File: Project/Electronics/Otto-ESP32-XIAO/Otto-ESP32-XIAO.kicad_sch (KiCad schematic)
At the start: 29 parts, among them J1 Conn_01x03, J10 Conn_01x02, J11 Conn_01x04, J12 OLED 0,91" - I2C (SKU21796), J13 MPU6050, J2 Conn_01x03, J3 Conn_01x03, J4 Conn_01x03, J5 Conn_01x03, J6 Conn_01x03, J7 Conn_01x04, J8 PCA9685, J9 Conn_01x04, SW1 SW_SPDT, U1 MOUDLE-SEEEDUINO-XIAO-ESP32C3, U2 R-78E5.0-1.0, U3 TMC2208_SILENTSTEPSTICK, U4 TMC2208_SILENTSTEPSTICK

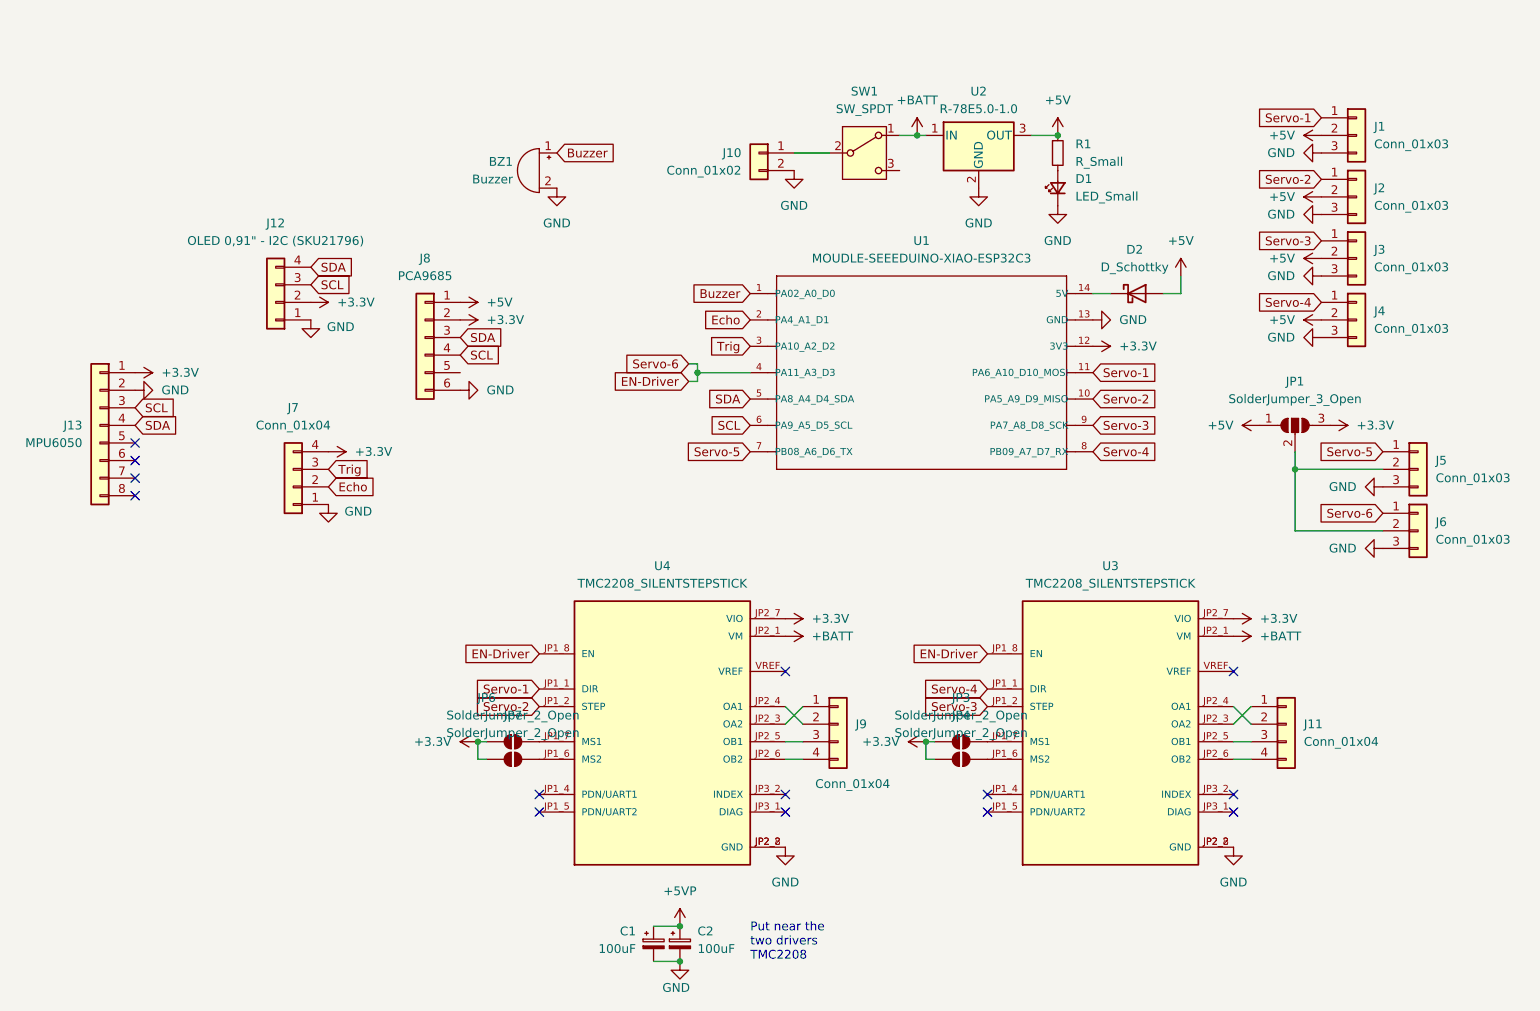
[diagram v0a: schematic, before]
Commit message: routing and documentation
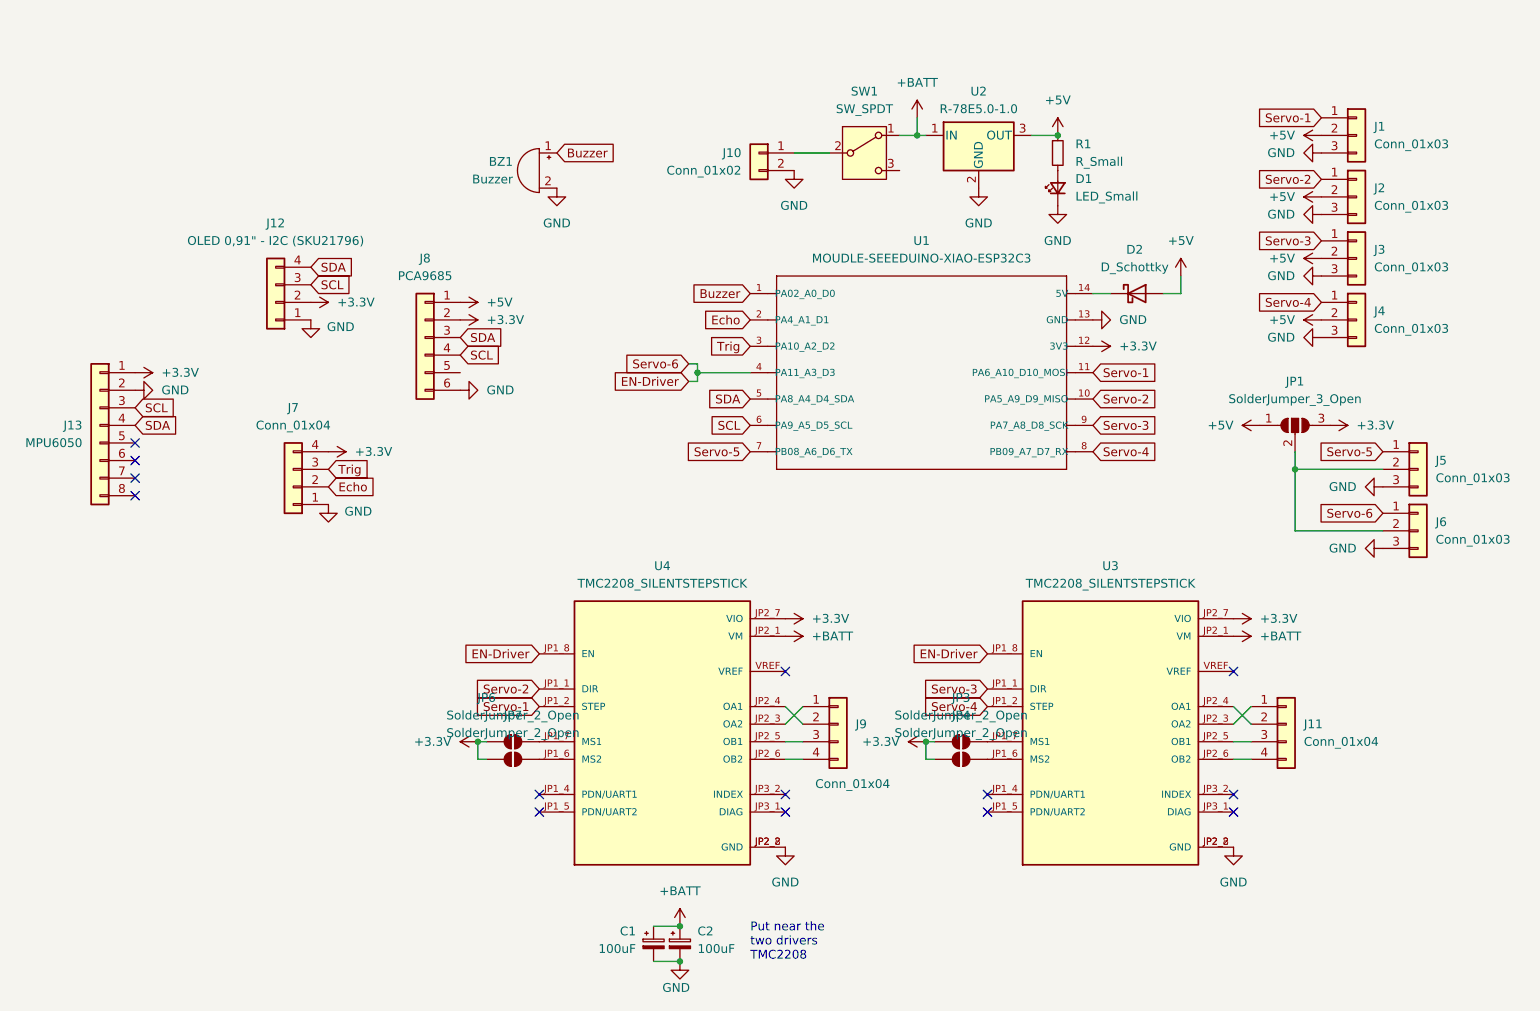
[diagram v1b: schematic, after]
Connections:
- net +5VP is gone; now on net +BATT: C1.1, C2.1
- net Servo-1: now also U4.JP1_2 (STEP); no longer U4.JP1_1 (DIR)
- net Servo-2: now also U4.JP1_1 (DIR); no longer U4.JP1_2 (STEP)
- net Servo-3: now also U3.JP1_1 (DIR); no longer U3.JP1_2 (STEP)
- net Servo-4: now also U3.JP1_2 (STEP); no longer U3.JP1_1 (DIR)
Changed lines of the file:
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@@
 	)
 	(junction
-		(at 111.76 168.91)
+		(at 114.3 88.9)
 		(diameter 0)
 		(color 0 0 0 0)
 	)
 	(junction
-		(at 114.3 88.9)
+		(at 200.66 102.87)
 		(diameter 0)
 		(color 0 0 0 0)
 	)
 	(junction
-		(at 200.66 102.87)
+		(at 146.05 54.61)
 		(diameter 0)
 		(color 0 0 0 0)
 	)
 	(junction
-		(at 146.05 54.61)
+		(at 111.76 168.91)
 		(diameter 0)
 		(color 0 0 0 0)
@@
 	(wire
 		(pts
-			(xy 146.05 54.61) (xy 147.32 54.61)
-		)
-		(stroke
-			(width 0)
-			(type default)
-		)
-	)
-	(wire
-		(pts
 			(xy 129.54 144.78) (xy 127 144.78)
 		)
@@
 	(wire
 		(pts
+			(xy 146.05 54.61) (xy 147.32 54.61)
+		)
+		(stroke
+			(width 0)
+			(type default)
+		)
+	)
+	(wire
+		(pts
 			(xy 147.32 142.24) (xy 147.32 144.78)
 		)
@@
 	(wire
 		(pts
+			(xy 143.51 54.61) (xy 146.05 54.61)
+		)
+		(stroke
+			(width 0)
+			(type default)
+		)
+	)
+	(wire
+		(pts
 			(xy 181.61 77.47) (xy 184.15 77.47)
 		)
@@
 	(wire
 		(pts
-			(xy 143.51 54.61) (xy 146.05 54.61)
+			(xy 107.95 168.91) (xy 111.76 168.91)
 		)
 		(stroke
@@
 	(wire
 		(pts
-			(xy 107.95 168.91) (xy 111.76 168.91)
+			(xy 191.77 139.7) (xy 194.31 137.16)
 		)
 		(stroke
@@
 	(wire
 		(pts
-			(xy 191.77 139.7) (xy 194.31 137.16)
+			(xy 114.3 88.9) (xy 114.3 90.17)
 		)
 		(stroke
@@
 	(wire
 		(pts
-			(xy 114.3 88.9) (xy 114.3 90.17)
+			(xy 200.66 111.76) (xy 200.66 102.87)
 		)
 		(stroke
@@
 	(wire
 		(pts
-			(xy 200.66 111.76) (xy 200.66 102.87)
+			(xy 82.55 144.78) (xy 83.82 144.78)
 		)
 		(stroke
@@
 	(wire
 		(pts
-			(xy 82.55 144.78) (xy 83.82 144.78)
+			(xy 191.77 137.16) (xy 194.31 139.7)
 		)
 		(stroke
@@
 	(wire
 		(pts
-			(xy 191.77 137.16) (xy 194.31 139.7)
+			(xy 146.05 52.07) (xy 146.05 54.61)
 		)
 		(stroke
@@
 		)
 	)
-	(global_label "Servo-4"
+	(global_label "Servo-3"
 		(shape input)
 		(at 156.21 134.62 180)
@@
 		)
 	)
-	(global_label "Servo-1"
+	(global_label "Servo-2"
 		(shape input)
 		(at 91.44 134.62 180)
@@
 		)
 	)
-	(global_label "Servo-2"
+	(global_label "Servo-1"
 		(shape input)
 		(at 91.44 137.16 180)
@@
 		)
 	)
-	(global_label "Servo-3"
+	(global_label "Servo-4"
 		(shape input)
 		(at 156.21 137.16 180)
@@
 	(symbol
 		(lib_id "power:+BATT")
-		(at 146.05 54.61 0)
+		(at 146.05 52.07 0)
 		(unit 1)
 		(exclude_from_sim no)
@@
 		(fields_autoplaced yes)
 		(property "Reference" "#PWR02"
-			(at 146.05 58.42 0)
+			(at 146.05 55.88 0)
 			(effects
 				(font
@@
 		)
 		(property "Value" "+BATT"
-			(at 146.05 49.53 0)
+			(at 146.05 46.99 0)
 			(effects
 				(font
@@
 		)
 		(property "Footprint" ""
-			(at 146.05 54.61 0)
+			(at 146.05 52.07 0)
 			(effects
 				(font
@@
 		)
 		(property "Datasheet" ""
-			(at 146.05 54.61 0)
+			(at 146.05 52.07 0)
 			(effects
 				(font
@@
 		)
 		(property "Description" "Power symbol creates a global label with name \"+BATT\""
-			(at 146.05 54.61 0)
+			(at 146.05 52.07 0)
 			(effects
 				(font
@@
 	)
 	(symbol
-		(lib_id "power:+5VP")
-		(at 111.76 168.91 0)
-		(unit 1)
-		(exclude_from_sim no)
-		(in_bom yes)
-		(on_board yes)
-		(dnp no)
-		(fields_autoplaced yes)
-		(property "Reference" "#PWR035"
-			(at 111.76 172.72 0)
-			(effects
-				(font
-					(size 1.27 1.27)
-				)
-				(hide yes)
-			)
-		)
-		(property "Value" "+5VP"
-			(at 111.76 163.83 0)
-			(effects
-				(font
-					(size 1.27 1.27)
-				)
-			)
-		)
-		(property "Footprint" ""
-			(at 111.76 168.91 0)
-			(effects
-				(font
-					(size 1.27 1.27)
-				)
-				(hide yes)
-			)
-		)
-		(property "Datasheet" ""
-			(at 111.76 168.91 0)
-			(effects
-				(font
-					(size 1.27 1.27)
-				)
-				(hide yes)
-			)
-		)
-		(property "Description" ""
-			(at 111.76 168.91 0)
-			(effects
-				(font
-					(size 1.27 1.27)
-				)
-				(hide yes)
-			)
-		)
-		(pin "1"
-		)
-		(instances
-			(project "Otto-ESP32-XIAO"
-				(path "/d2682c99-4285-4c0b-9e61-08b763b3ce0d"
-					(reference "#PWR035")
-					(unit 1)
-				)
-			)
-		)
-	)
-	(symbol
 		(lib_id "Connector_Generic:Conn_01x03")
 		(at 209.55 54.61 0)
@@
 					(unit 1)
 				)
+			)
+		)
+	)
+	(symbol
+		(lib_id "power:+BATT")
+		(at 111.76 168.91 0)
+		(unit 1)
+		(exclude_from_sim no)
+		(in_bom yes)
+		(on_board yes)
+		(dnp no)
+		(fields_autoplaced yes)
+		(property "Reference" "#PWR041"
+			(at 111.76 172.72 0)
+			(effects
+				(font
+					(size 1.27 1.27)
+				)
+				(hide yes)
+			)
+		)
+		(property "Value" "+BATT"
+			(at 111.76 163.83 0)
+			(effects
+				(font
+					(size 1.27 1.27)
+				)
+			)
+		)
+		(property "Footprint" ""
+			(at 111.76 168.91 0)
+			(effects
+				(font
+					(size 1.27 1.27)
+				)
+				(hide yes)
+			)
+		)
+		(property "Datasheet" ""
+			(at 111.76 168.91 0)
+			(effects
+				(font
+					(size 1.27 1.27)
+				)
+				(hide yes)
+			)
+		)
+		(property "Description" "Power symbol creates a global label with name \"+BATT\""
+			(at 111.76 168.91 0)
+			(effects
+				(font
+					(size 1.27 1.27)
+				)
+				(hide yes)
+			)
+		)
+		(pin "1"
+		)
+		(instances
+			(project "Otto-ESP32-XIAO"
+				(path "/d2682c99-4285-4c0b-9e61-08b763b3ce0d"
+					(reference "#PWR041")
+					(unit 1)
+				)

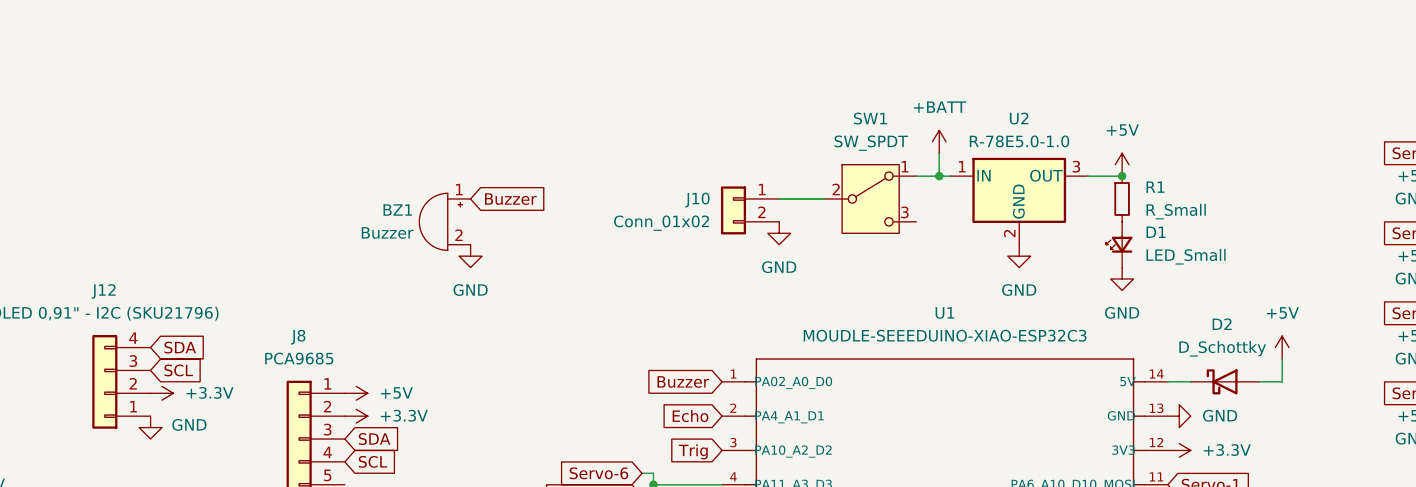
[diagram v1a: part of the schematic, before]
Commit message: New PCB lite version
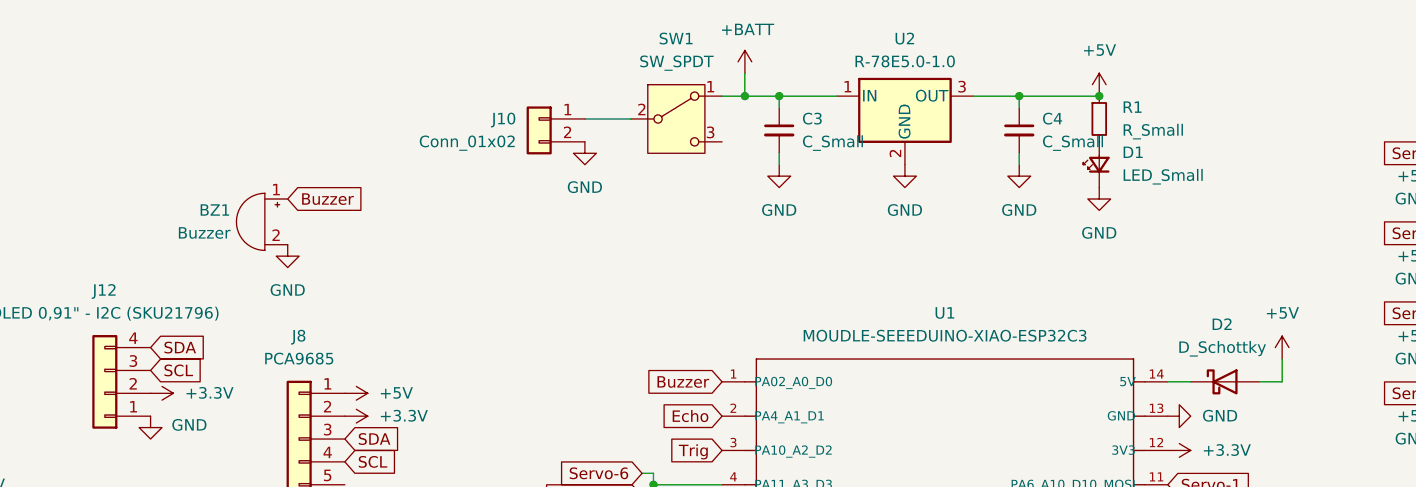
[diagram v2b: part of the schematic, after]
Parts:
- added C3, C4: C_Small, Capacitor_THT:C_Disc_D6.0mm_W2.5mm_P5.00mm, symbol Device:C_Small
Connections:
- net +5V: now also C4.1
- net +BATT: now also C3.1
- net GND: now also C3.2, C4.2
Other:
- moved on the sheet: BZ1, D1, J10, R1, SW1, U2
